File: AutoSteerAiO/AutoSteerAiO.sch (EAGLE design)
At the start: 85 parts, among them J4 CONNECTOR 1x5 PINS, K4 CB1A-P-12V, T1 BC547, U1 VX7805-1000

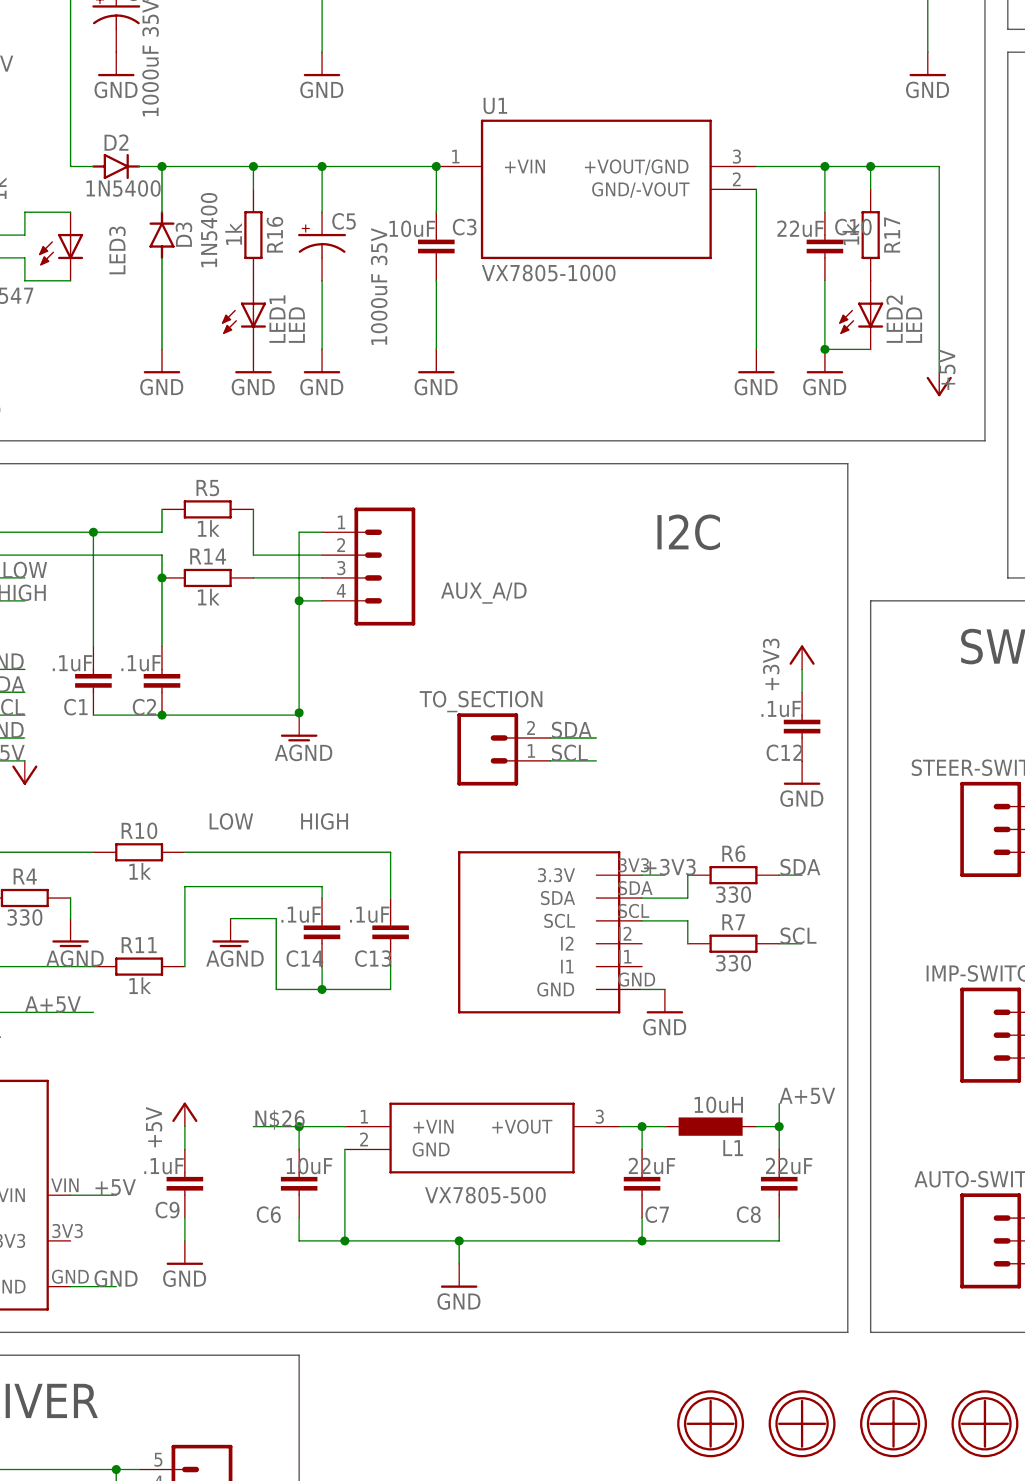
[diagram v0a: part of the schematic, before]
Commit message: Add files via upload
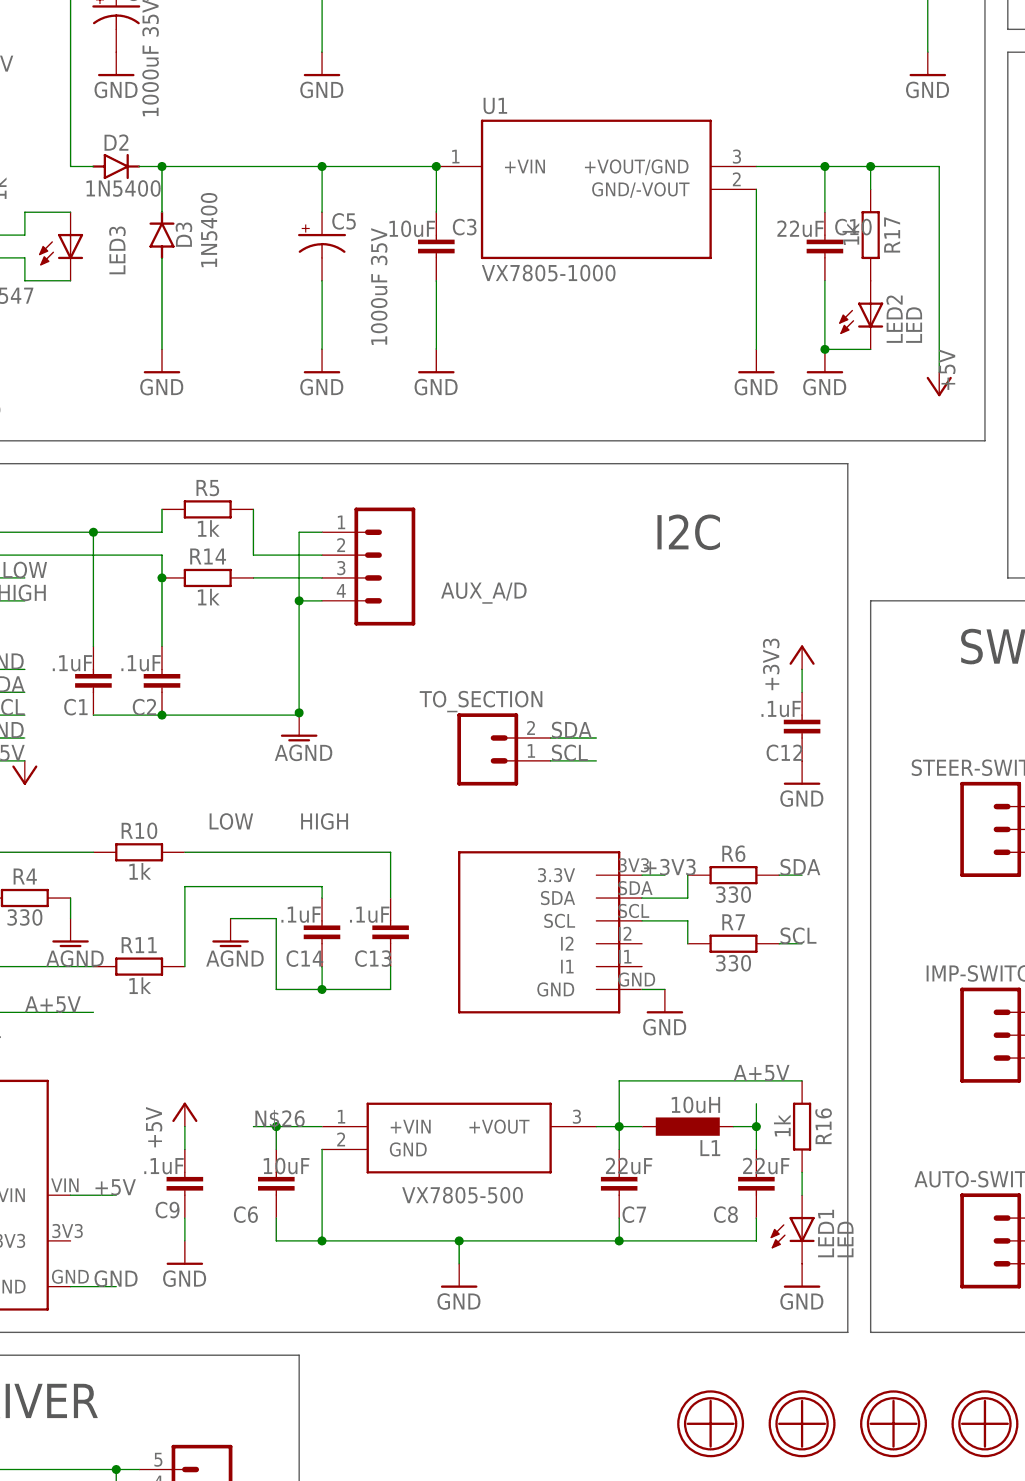
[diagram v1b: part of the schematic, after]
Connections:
- net N$25: now also R16.1
- net N$26: no longer R16.1
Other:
- moved on the sheet: C6, C7, C8, L1, LED1, R16
